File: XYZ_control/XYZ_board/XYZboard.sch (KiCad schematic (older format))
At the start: 75 parts, among them J1 DB9 X, J10 DB9 Y, J11 Gnd Out, J12 Sensor X, J13 Sensor Y, J14 Sensor Z, J15 DB9 Z, J2 Control X, J3 Control Y, J4 Control Z, J5 PWR IN, J6 Settings X, J7 Settings Y, J8 Settings Z, J9 Vcc Out, U1 LM317MSTT3G_Voltage_Regulator, U2 A4988_stepper_driver, U3 A4988_stepper_driver, U4 A4988_stepper_driver

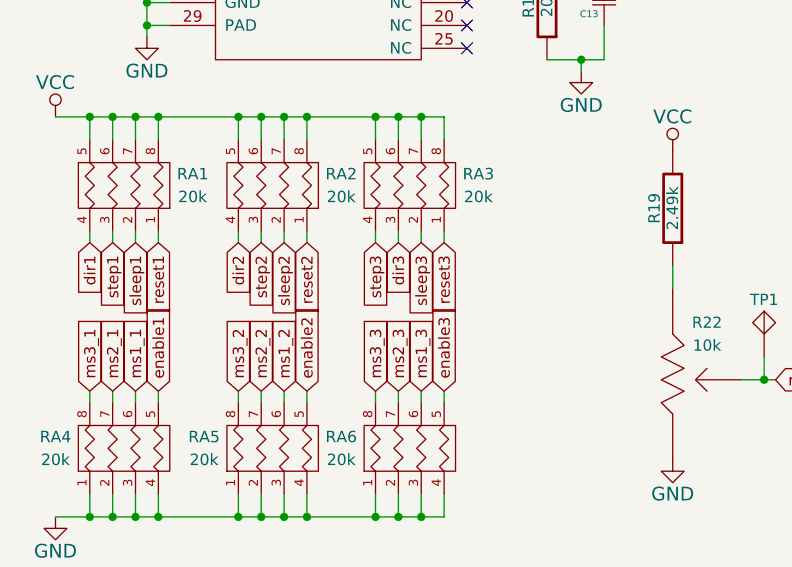
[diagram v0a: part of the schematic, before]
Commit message: xyz board progress
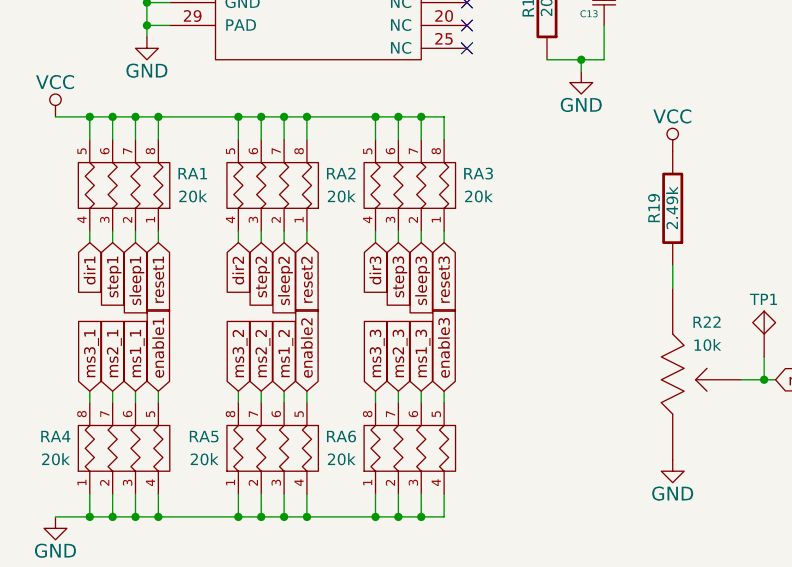
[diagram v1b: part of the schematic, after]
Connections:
- net dir3: now also RA3.4 (P4); no longer RA3.3 (P3)
- net step3: now also RA3.3 (P3); no longer RA3.4 (P4)
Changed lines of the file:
@@
 Text GLabel 1800 6400 3    49   Input ~ 0
 sleep2
+Text GLabel 2300 6400 3    49   Input ~ 0
+step3
 Text GLabel 2200 6400 3    49   Input ~ 0
-step3
-Text GLabel 2300 6400 3    49   Input ~ 0
 dir3
 Text GLabel 2500 6400 3    49   Input ~ 0
